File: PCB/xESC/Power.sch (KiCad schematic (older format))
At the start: 21 parts, among them U2 TMC6100-LA, U3 LMV321

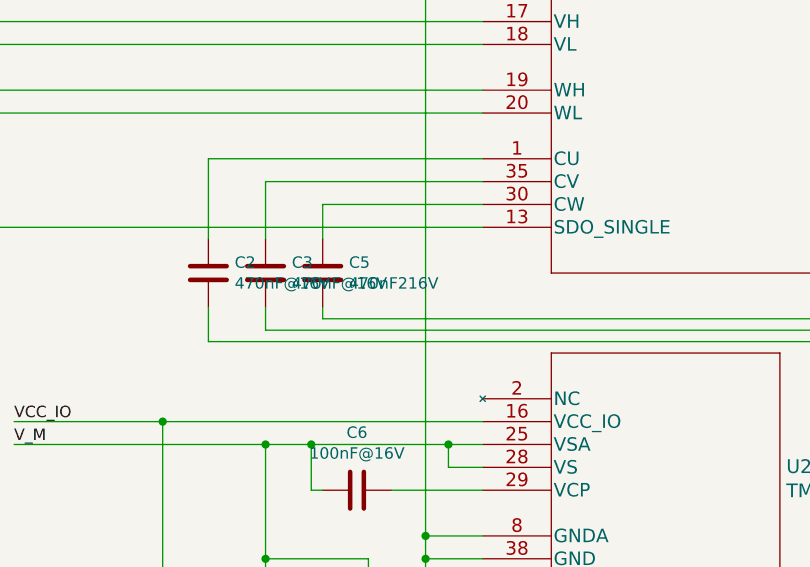
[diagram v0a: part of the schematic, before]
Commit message: wip
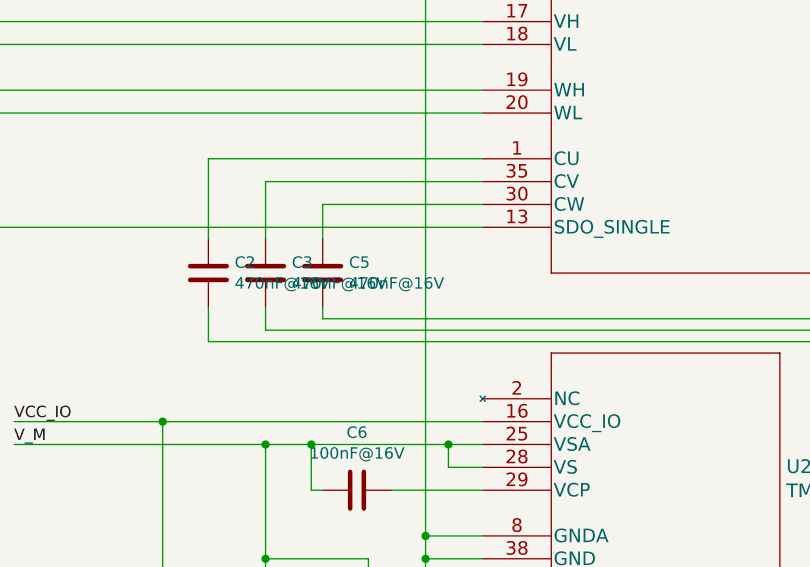
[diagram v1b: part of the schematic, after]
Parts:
- C5: value 470nF216V -> 470nF@16V
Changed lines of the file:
@@
 P 2900 3950
 F 0 "C5" H 3015 3996 50  0000 L CNN
-F 1 "470nF216V" H 3015 3905 50  0000 L CNN
+F 1 "470nF@16V" H 3015 3905 50  0000 L CNN
 F 2 "Capacitor_SMD:C_0805_2012Metric_Pad1.18x1.45mm_HandSolder" H 2938 3800 50  0001 C CNN
 F 3 "~" H 2900 3950 50  0001 C CNN
